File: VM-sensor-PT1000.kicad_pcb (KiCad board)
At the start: 2 copper layers, 25.4 x 21.6 mm, 17 parts, among them P1 PT100, P2 ADC, P3 PWR, U1 AMS1117, U2 MCP6001

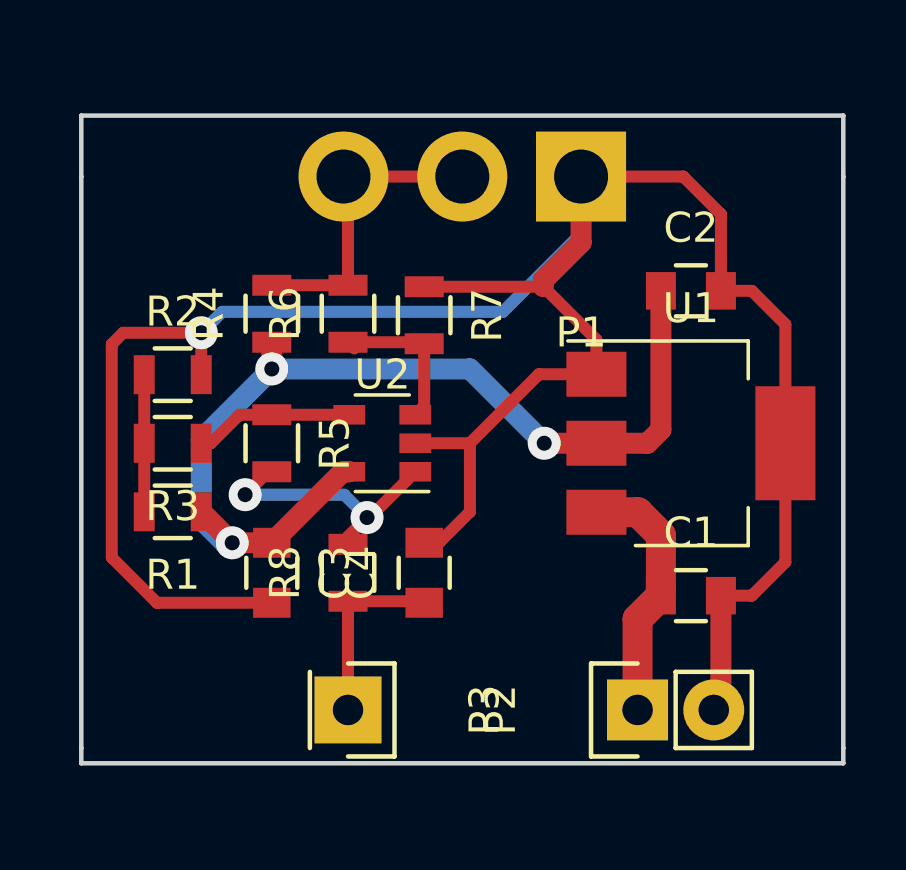
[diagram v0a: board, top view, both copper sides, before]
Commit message: Completed PCB
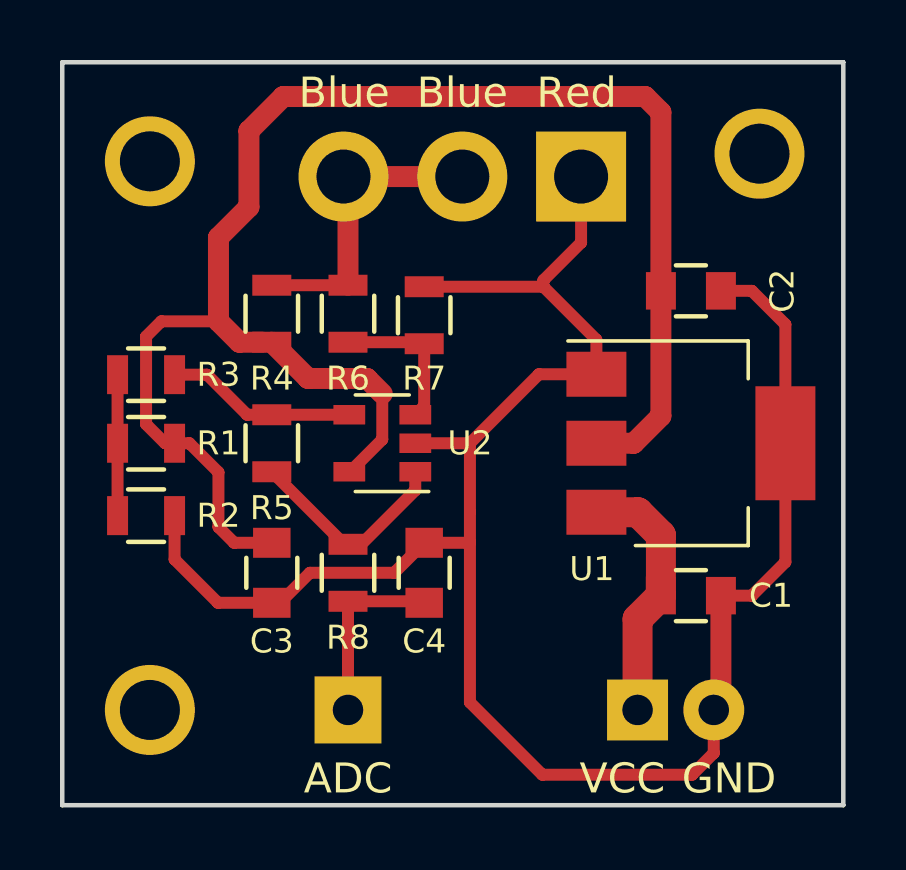
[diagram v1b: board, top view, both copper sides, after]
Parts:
- added REF**: SolderWirePad_single_1-2mmDrill, Wire_Pads:SolderWirePad_single_1-2mmDrill, F.Cu at (116.6, 63.0)
- added REF**: SolderWirePad_single_1-2mmDrill, Wire_Pads:SolderWirePad_single_1-2mmDrill, F.Cu at (116.6, 81.3)
- added REF**: SolderWirePad_single_1-2mmDrill, Wire_Pads:SolderWirePad_single_1-2mmDrill, F.Cu at (136.9, 62.7)
- moved R2 4.78 mm to (116.5, 74.8)
- moved R1 2.45 mm to (116.5, 72.4)
- moved R3 2.45 mm to (116.5, 70.1)
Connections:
- net /Red renamed /Blue
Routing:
- net +3V3: track 33.4 -> 55.9 mm, vias 3 -> 0
- net GND: track 81.6 -> 68.1 mm, vias 1 -> 0
- net Net-(R5-Pad2): track 8.98 -> 7.27 mm, vias 2 -> 0
- net Net-(R3-Pad1): track 5.33 -> 6.38 mm
- added copper zone on F.Cu, net GND
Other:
- board size 25.4 x 21.6 mm -> 26 x 24.8 mm
- net class Default: trace_width 0.4 -> 0.7
- board text added: "ADC"
- board text added: "Blue"
- board text added: "GND"
- board text added: "Red"
- board text added: "VCC"
